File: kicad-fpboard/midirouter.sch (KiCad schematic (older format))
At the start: 43 parts, among them J1 MIDI_IN_1, J10 Conn_01x08, J2 MIDI_IN_2, J3 MIDI_IN_3, J4 MIDI_IN_4, J5 Conn_01x08, J6 MIDI_OUT_1, J7 MIDI_OUT_2, J8 MIDI_OUT_3, J9 MIDI_OUT_4, U1 PC847

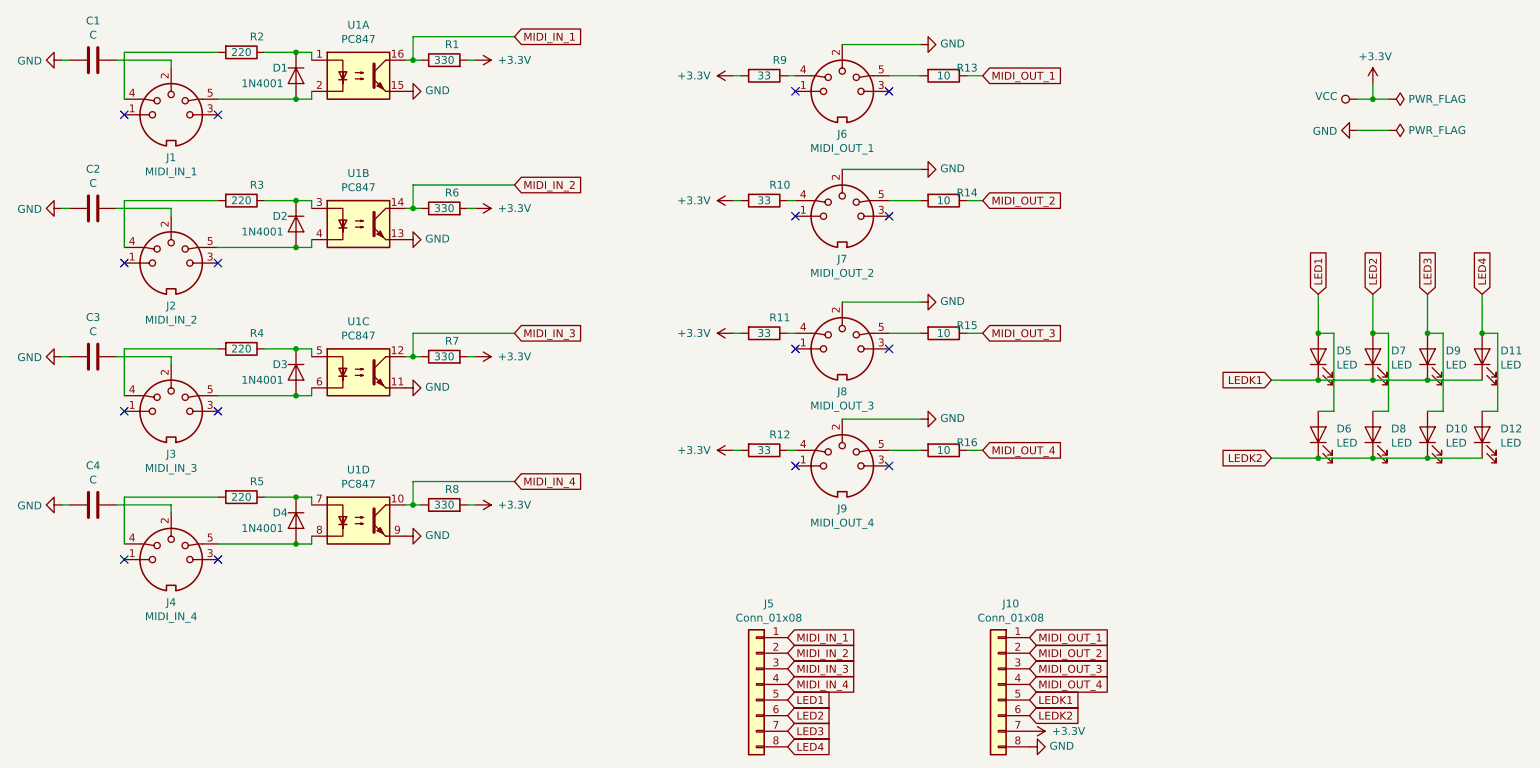
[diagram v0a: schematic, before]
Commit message: Work on schematics and pcbs.
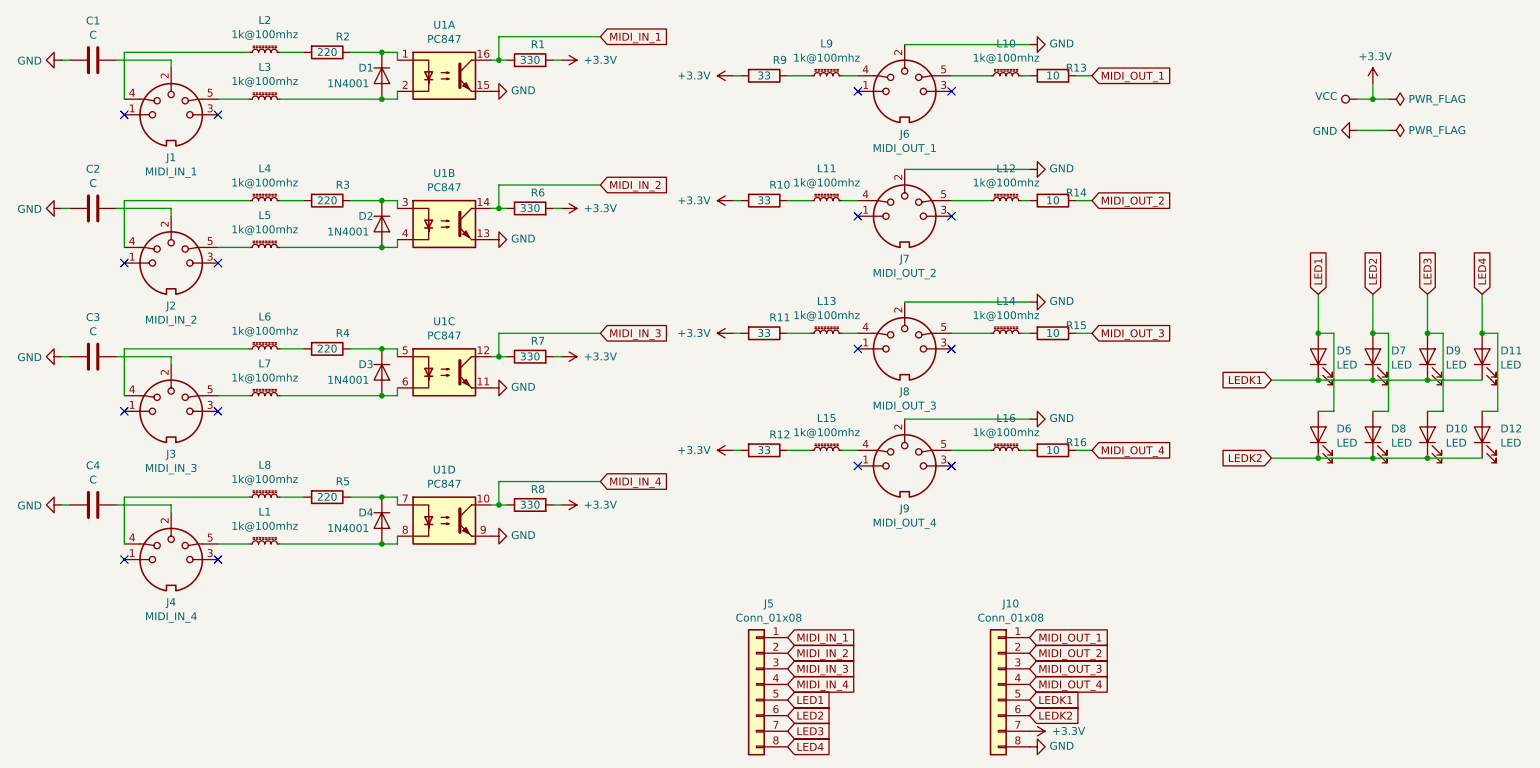
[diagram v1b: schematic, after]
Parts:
- added L1, L10, L11, L12, L13, L14, L15, L16, L2, L3, L4, L5, L6, L7, L8, L9: 1k@100mhz, Inductor_SMD:L_0603_1608Metric_Pad1.05x0.95mm_HandSolder, symbol Device:L_Core_Ferrite_Small
- C1, C2, C3, C4: footprint Capacitor_SMD:C_1206_3216Metric_Pad1.42x1.75mm_HandSolder -> Capacitor_SMD:C_0805_2012Metric
- D1, D2, D3, D4: footprint Diode_SMD:D_1206_3216Metric_Pad1.42x1.75mm_HandSolder -> Diode_SMD:D_0805_2012Metric
- R1, R10, R11, R12, R13, R14, R15, R16, R2, R3, R4, R5, R6, R7, R8, R9: footprint Resistor_SMD:R_1206_3216Metric_Pad1.42x1.75mm_HandSolder -> Resistor_SMD:R_0805_2012Metric
- U1: footprint Package_SO:SOP-16_7.5x10.4mm_P1.27mm -> Package_SO:SOP-16_4.4x10.4mm_P1.27mm
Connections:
- net at D1.2 (A), U1.2: now also L3.2; no longer J1.5
- net at J1.4: now also L2.1; no longer R2.2
- net at R13.2: now also L10.2; no longer J6.5
- net at R14.2: now also L12.2; no longer J7.5
- net at R15.2: now also L14.2; no longer J8.5
- net at R16.2: now also L16.2; no longer J9.5
- net at J6.4: now also L9.2; no longer R9.1
- net at J7.4: now also L11.2; no longer R10.1
- net at J8.4: now also L13.2; no longer R11.1
- net at J9.4: now also L15.2; no longer R12.1
- net at D2.2 (A), U1.4: now also L5.2; no longer J2.5
- net at J2.4: now also L4.1; no longer R3.2
- net at D3.2 (A), U1.6: now also L7.2; no longer J3.5
- net at J3.4: now also L6.1; no longer R4.2
- net at D4.2 (A), U1.8: now also L1.2; no longer J4.5
- net at J4.4: now also L8.1; no longer R5.2
- new net: J1.5, L3.1
- new net: L2.2, R2.2
- new net: J6.5, L10.1
- new net: J7.5, L12.1
- new net: J8.5, L14.1
- new net: J9.5, L16.1
- new net: L9.1, R9.1
- new net: L11.1, R10.1
- new net: L13.1, R11.1
- new net: L15.1, R12.1
- new net: J2.5, L5.1
- new net: L4.2, R3.2
- new net: J3.5, L7.1
- new net: L6.2, R4.2
- new net: J4.5, L1.1
- new net: L8.2, R5.2
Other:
- moved on the sheet: D1, D2, D3, D4, J6, J7, J8, J9, R1, R13, R14, R15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
